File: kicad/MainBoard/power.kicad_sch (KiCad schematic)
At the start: 63 parts, among them J16 Conn_01x02_Female, J20 USB_C_Receptacle, Q16 AO3401A, Q17 AO3401A, SW1 Power switch, U13 BQ27441-G1, U14 HY2111-GB, U15 FS8205A, U16 TP4056, U17 TPS61088

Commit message: update out of stock 0.5R resistor C705591 to be C175573 instead
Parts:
- R132: LCSC C705591 -> C175573
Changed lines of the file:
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@@
       (effects (font (size 1.27 1.27)) hide)
     )
-    (property "LCSC" "C705591" (id 4) (at 121.92 23.495 0)
+    (property "LCSC" "C175573" (id 4) (at 121.92 23.495 0)
       (effects (font (size 1.27 1.27)) hide)
     )

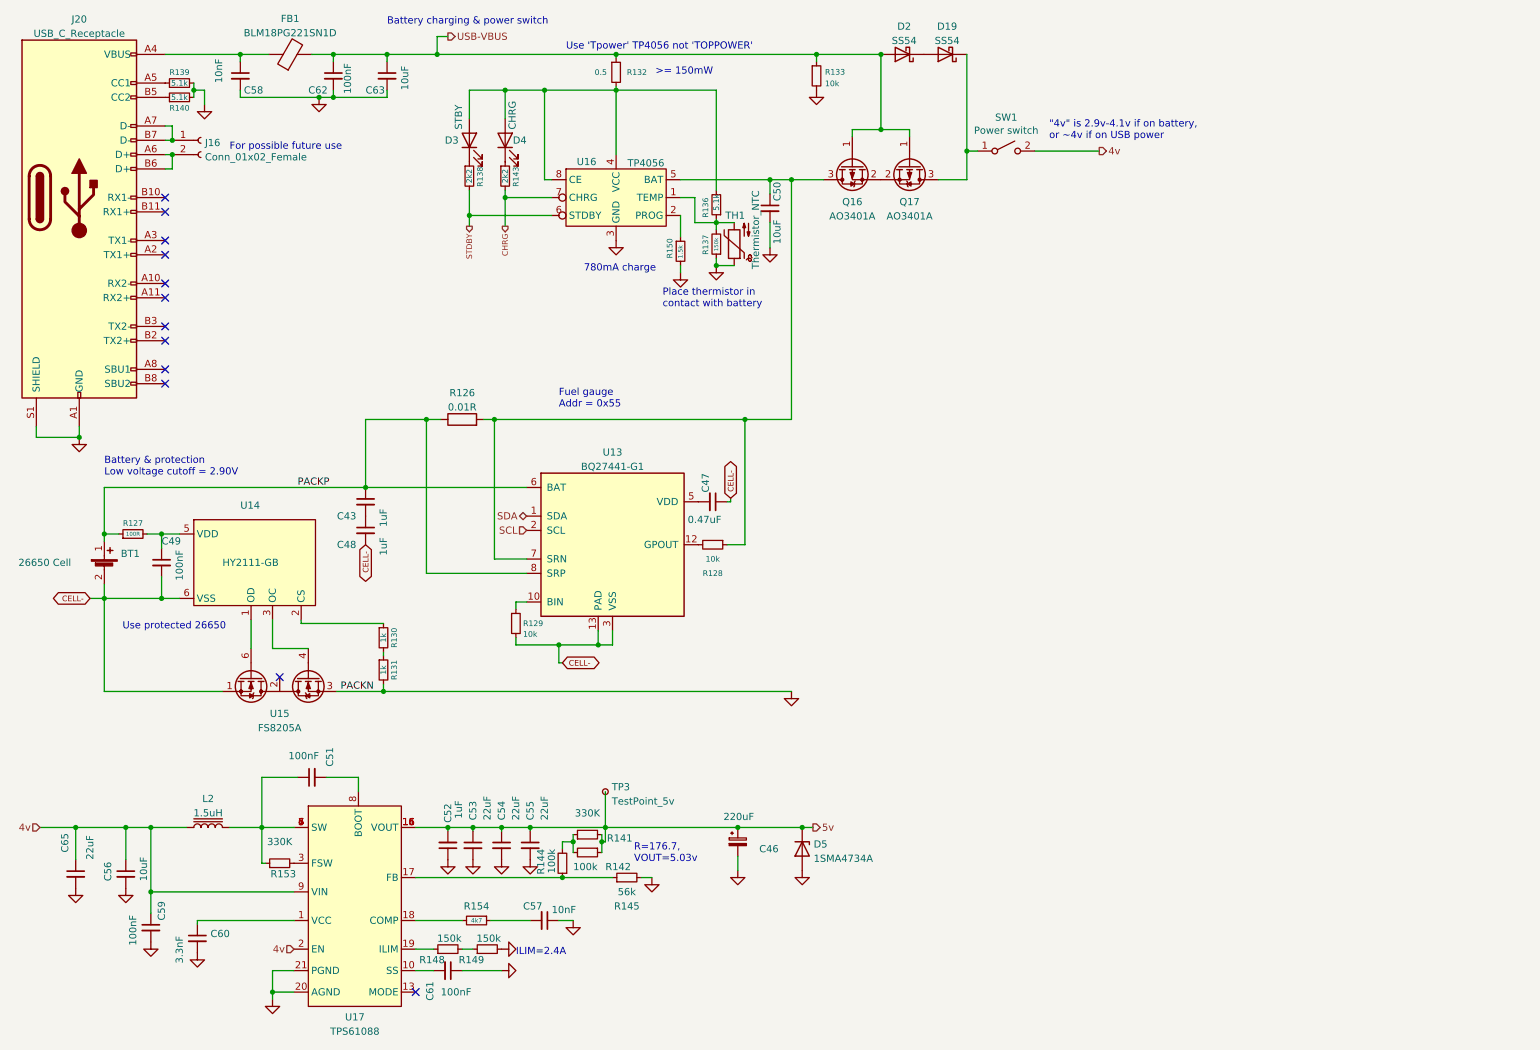
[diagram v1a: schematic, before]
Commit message: Add PCB v2.3 kicad project files + gerbers
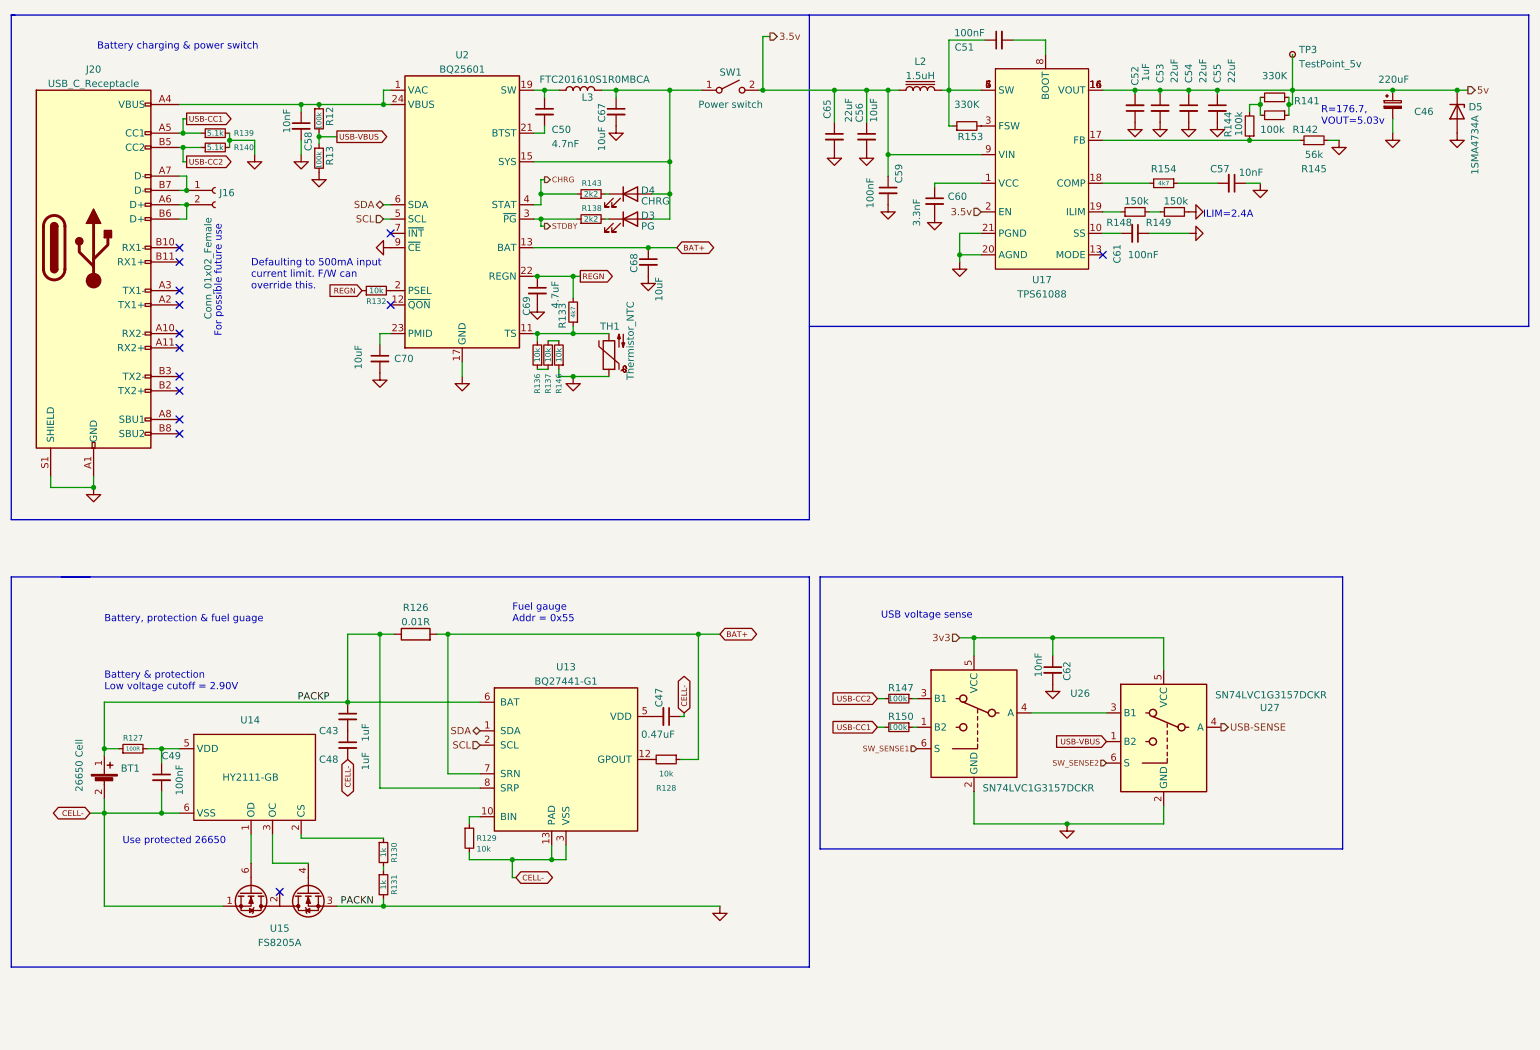
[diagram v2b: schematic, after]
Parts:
- removed C63: 10uF, Capacitor_SMD:C_0603_1608Metric_Pad1.08x0.95mm_HandSolder, symbol Device:C_Small
- removed D19, D2: SS54, Diode_SMD:D_SMA_Handsoldering, symbol Device:D_Schottky
- removed FB1: BLM18PG221SN1D, Inductor_SMD:L_0603_1608Metric_Pad1.05x0.95mm_HandSolder, symbol Device:FerriteBead
- removed Q16, Q17: AO3401A, Package_TO_SOT_SMD:SOT-23_Handsoldering, symbol Transistor_FET:AO3401A
- removed U16: TP4056, Package_SO:SOP-8_3.76x4.96mm_P1.27mm, symbol ZcLib:TP4056
- added C67, C68, C70: 10uF, Capacitor_SMD:C_0603_1608Metric_Pad1.08x0.95mm_HandSolder, symbol Device:C_Small
- added C69: 4.7uF, Capacitor_SMD:C_0603_1608Metric_Pad1.08x0.95mm_HandSolder, symbol Device:C_Small
- added L3: FTC201610S1R0MBCA, ProjLib:FTC201610S, symbol Device:L
- added R12, R13, R147: 100k, Resistor_SMD:R_0603_1608Metric_Pad0.98x0.95mm_HandSolder, symbol Device:R_Small
- added R146: 10k, Resistor_SMD:R_0603_1608Metric_Pad0.98x0.95mm_HandSolder, symbol Device:R_Small
- added U2: BQ25601, Package_DFN_QFN:Texas_S-PWQFN-N24_EP2.7x2.7mm_ThermalVias, symbol Battery_Management:BQ25601
- added U26, U27: SN74LVC1G3157DCKR, Package_TO_SOT_SMD:SOT-363_SC-70-6_Handsoldering, symbol zclib:SN74LVC1G3157DCKR
- C50: value 10uF -> 4.7nF; LCSC C19702 -> C53987
- C62: value 100nF -> 10nF; LCSC C14663 -> C57112
- D3: value STBY -> PG
- R132: value 0.5 -> 10k; footprint Resistor_SMD:R_1218_3246Metric_Pad1.22x4.75mm_HandSolder -> Resistor_SMD:R_0603_1608Metric_Pad0.98x0.95mm_HandSolder; LCSC C175573 -> C25804
- R133: value 10k -> 4k7; LCSC C25804 -> C23162
- R136: value 5.1k -> 10k; LCSC C23186 -> C25804
- R137: value 150k -> 10k; LCSC C22807 -> C25804
- R150: value 1.5k -> 100k; LCSC C22843 -> C25803
- TH1: footprint Connector_PinSocket_2.54mm:PinSocket_1x02_P2.54mm_Vertical -> Connector_PinHeader_2.54mm:PinHeader_1x02_P2.54mm_Vertical
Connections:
- net CHRG: now also R143.1, U2.4 (STAT); no longer R143.2
- net GND: now also C67.2, C68.2, C69.2, C70.2, R13.2, R146.1, U2.17 (GND), U2.18 (GND), U2.25 (GND), U2.9 (~{CE}), U26.2 (GND), U27.2 (GND); no longer C50.2, R133.2, R137.1, R150.2
- net SCL: now also U2.5 (SCL)
- net SDA: now also U2.6 (SDA)
- net STDBY: now also R138.1, U2.3 (~{PG}); no longer R138.2
- net USB-VBUS: now also R12.2, R13.1, U27.1 (B2); no longer C62.1, R132.1, R133.1
- net USB-CC2: now reaches J20.B5 (CC2), R140.1
- net USB-CC2: now also R147.2
- net at D3.2 (A), D4.2 (A): now also SW1.1 (A), C67.1, L3.2, U2.15 (SYS), U2.16 (SYS); no longer R132.2, R136.2
- net at D3.1 (K): now also R138.2; no longer R138.1
- net BAT+: now reaches R126.2, R128.1, U13.7 (SRN)
- net BAT+: now also C68.1, U2.13 (BAT), U2.14 (BAT); no longer C50.1
- net at D4.1 (K): now also R143.2; no longer R143.1
- net at C58.1, J20.A4 (VBUS), J20.A9 (VBUS)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: now also R12.1, U2.1 (VAC), U2.24 (VBUS)
- net USB-CC1: now reaches J20.A5 (CC1), R139.1
- net USB-CC1: now also R150.2
- net at R150.1: now also U26.1 (B2)
- net 4v renamed 3.5v
- new net: R147.1, U26.3 (B1)
- new net: U26.4 (A), U27.3 (B1)
- new net: R136.1, R137.1
- new net: R133.1, R136.2, TH1.2, U2.11 (TS)
- new net: R137.2, R146.2
- new net: R132.2, U2.2 (PSEL)
- new net: C70.1, U2.23 (PMID)
- new net: C50.1, L3.1, U2.19 (SW), U2.20 (SW)
- new net: C50.2, U2.21 (BTST)
- new net 3v3: C62.1, U26.5 (VCC), U27.5 (VCC)
- new net REGN: C69.1, R132.1, R133.2, U2.22 (REGN)
- new net SW_SENSE1: U26.6 (S)
- new net SW_SENSE2: U27.6 (S)
- new net USB-SENSE: U27.4 (A)
- no-connect marks 12 -> 14
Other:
- note added: "Battery, protection & fuel guage"
- note added: "Defaulting to 500mA input current limit. F/W can override this."
- note added: "USB voltage sense"
- note removed: ""4v" is 2.9v-4.1v if on battery, or ~4v if on USB power"
- note removed: "780mA charge"
- note removed: ">= 150mW"
- note removed: "Place thermistor in contact with battery"
- note removed: "Use 'Tpower' TP4056 not 'TOPPOWER'"
- moved on the sheet: BT1, C43, C46, C47, C48, C49, C51, C52, C53, C54, C55, C56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
